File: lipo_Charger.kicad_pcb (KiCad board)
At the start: 4 copper layers, 82.7 x 80.4 mm, 111 parts, among them J1 XT60PW-M, J2 Conn_01x01, J3 balance_plug_4s, J4 Conn_01x05, J5 Conn_01x04, J6 Conn_01x01, J7 Conn_01x07, J8 Conn_01x04, Q1 NX7002AK_215(nch low power), Q2 NVTFS010N10MCLTAG(high power), Q3 NVTFS010N10MCLTAG(high power), Q4 NVTFS010N10MCLTAG(high power), Q5 NVTFS010N10MCLTAG(high power), Q6 NX7002AK_215(nch low power), Q7 NX7002AK_215(nch low power), Q8 NX7002AK_215(nch low power), U1 BQ25703ARSNR

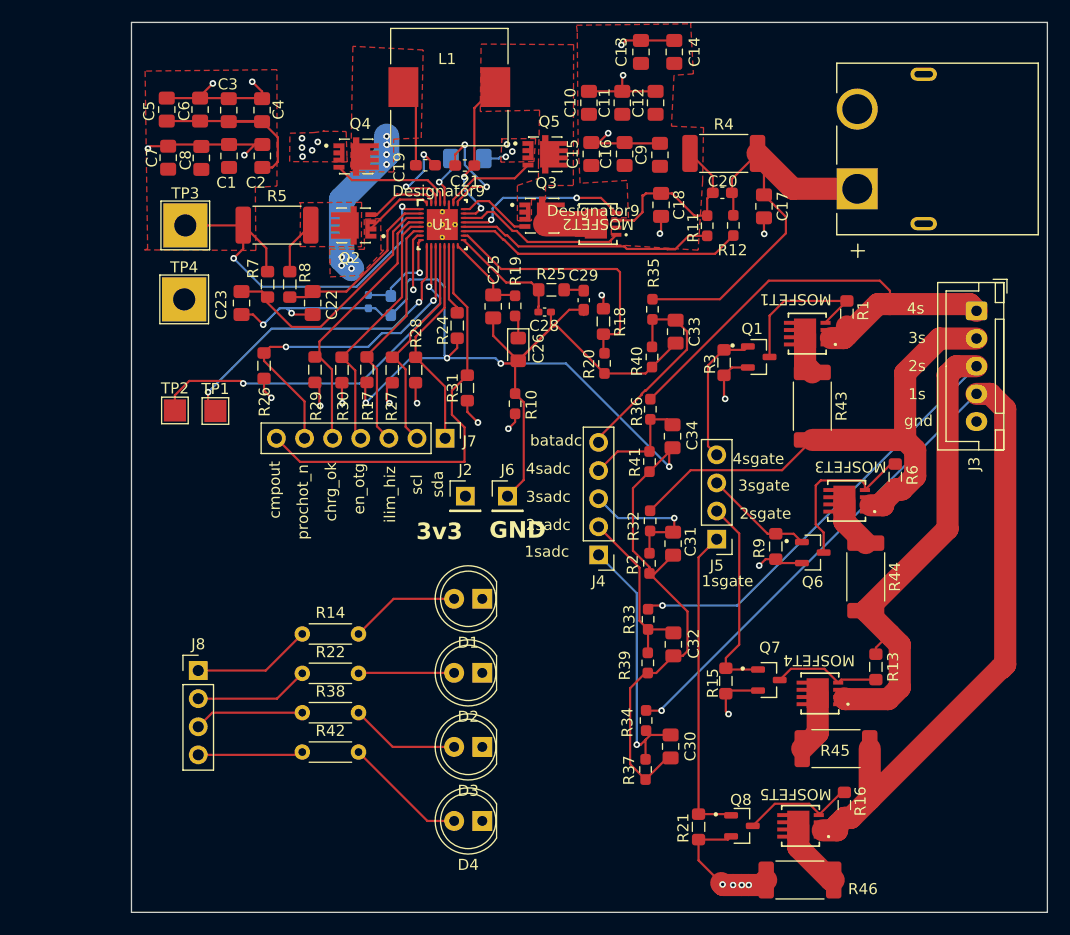
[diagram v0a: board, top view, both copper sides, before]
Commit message: final correction has been ready to order
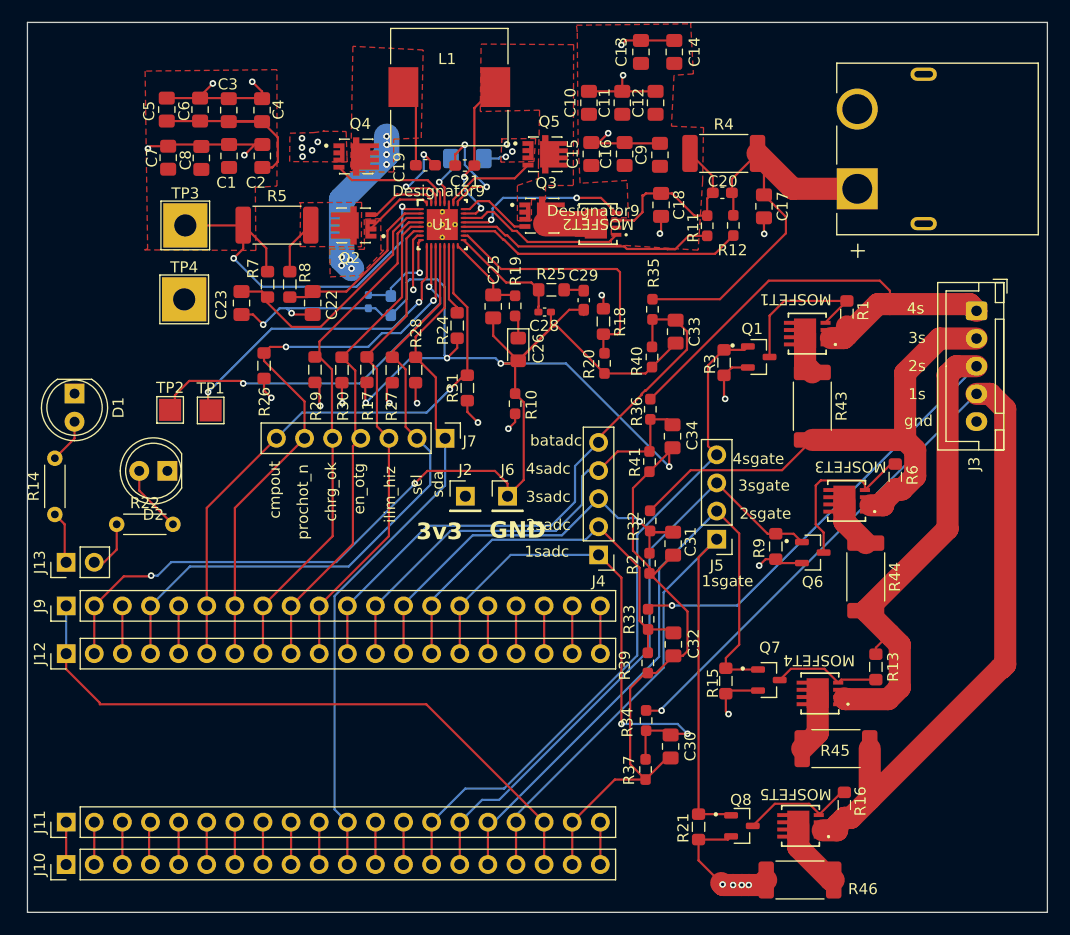
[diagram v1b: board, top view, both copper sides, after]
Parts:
- removed D3, D4: LED, LED_THT:LED_D5.0mm
- removed J8: Conn_01x04, Connector_PinHeader_2.54mm:PinHeader_1x04_P2.54mm_Vertical
- removed R38, R42: R, Resistor_THT:R_Axial_DIN0204_L3.6mm_D1.6mm_P5.08mm_Horizontal
- added J10: Conn_01x20, Connector_PinHeader_2.54mm:PinHeader_1x20_P2.54mm_Vertical, F.Cu at (90.0, 130.4)
- added J11: Conn_01x20, Connector_PinHeader_2.54mm:PinHeader_1x20_P2.54mm_Vertical, F.Cu at (90.0, 126.6)
- added J12: Conn_01x20, Connector_PinHeader_2.54mm:PinHeader_1x20_P2.54mm_Vertical, F.Cu at (90.0, 111.4)
- added J13: Conn_01x02, Connector_PinHeader_2.54mm:PinHeader_1x02_P2.54mm_Vertical, F.Cu at (90.0, 103.1)
- added J9: Conn_01x20, Connector_PinHeader_2.54mm:PinHeader_1x20_P2.54mm_Vertical, F.Cu at (90.0, 107.1)
- moved D1 41.2 mm to (90.8, 87.9), turned to -90 degrees
- moved D2 33.8 mm to (99.2, 94.9)
- moved R14 24.8 mm to (89.0, 98.8), turned to 90 degrees
- moved R22 21.5 mm to (94.6, 99.7)
- moved TP1 0.43 mm to (103.1, 89.4)
- moved TP2 0.43 mm to (99.4, 89.4)
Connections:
- net /PROCHOT_N renamed /PB0
- net /SCL renamed /PB10
- net /SDA renamed /PB3
- net Net-(J5-Pin_1) renamed /1SGATE
- net Net-(J5-Pin_2) renamed /2SGATE
- net Net-(J5-Pin_3) renamed /3SGATE
- net Net-(J5-Pin_4) renamed /4SGATE
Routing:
- net GNDA: track 161.4 -> 221.8 mm, vias 6 -> 8
- net /5V: track 0.00 -> 58.5 mm
- net /4SGATE: track 12.7 -> 62.4 mm
- net /3SGATE: track 9.91 -> 54.9 mm
- net /PB3: track 19.6 -> 62.7 mm
- net /2SGATE: track 18.5 -> 59.3 mm
- net /PB10: track 20.1 -> 58.9 mm
- net /1SGATE: track 28.5 -> 65.4 mm
- net /BAT_adc: track 19.4 -> 54.5 mm
- net /CELL_4S_adc: track 10.5 -> 41.5 mm
- net /CELL_3S_adc: track 13.0 -> 38.1 mm
- net /CELL_1S_adc: track 24.3 -> 47.8 mm, vias 1 -> 2
- net /CELL_2S_adc: track 15.7 -> 38.3 mm
- net /EN_OTG: track 23.3 -> 45.4 mm
- net /ILIM_HIZ: track 21.9 -> 44.0 mm
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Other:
- board size 82.7 x 80.4 mm -> 92.1 x 80.4 mm
